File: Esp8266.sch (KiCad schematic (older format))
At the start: 32 parts, among them P1 AUTO-PROGRAM JUMPER, P2 CONN_02X10, P3 LiPo, P5 OLED_I2C, P6 USB Serial, SW1 RESET, U1 SPX1117, U2 MCP73831, U3 ESP-12E

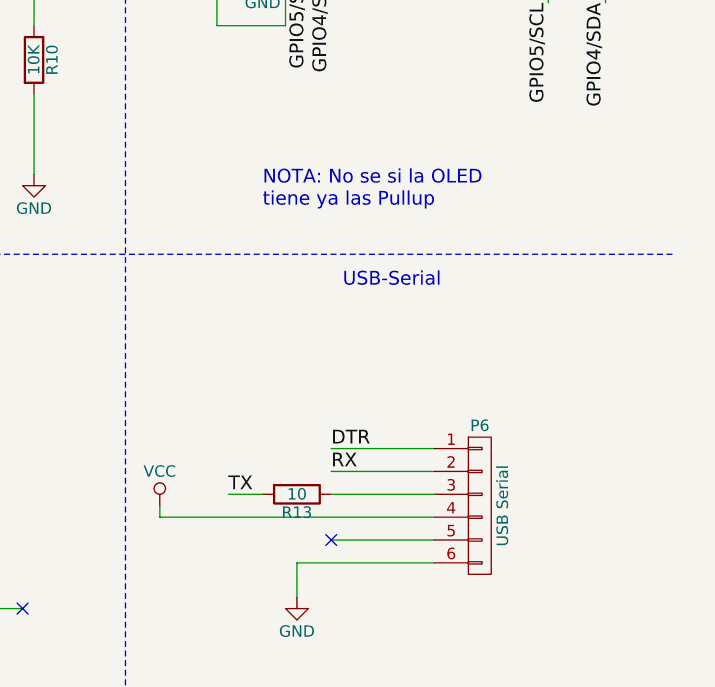
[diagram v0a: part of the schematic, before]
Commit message: Version 007-121215
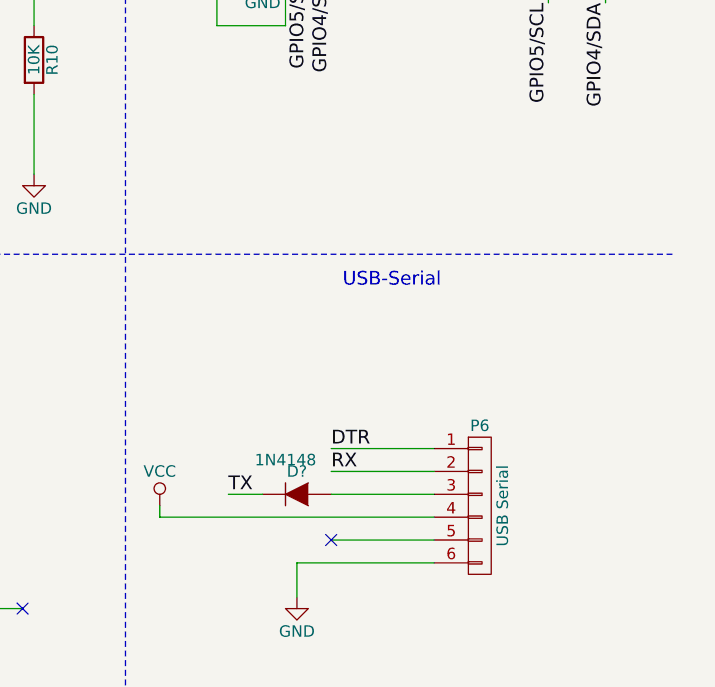
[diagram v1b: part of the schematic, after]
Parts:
- removed R13: 10, symbol R
- added D?: 1N4148, symbol D
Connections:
- net TX: now also D?.1 (K)
- net at P6.3 (P3): now also D?.2 (A)
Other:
- note removed: "NOTA: No se si la OLED \ntiene ya las Pullup"
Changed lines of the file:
@@
 Sheet 2 3
 Title "BadgeInventorsCon"
-Date "2015-12-07"
-Rev "0.06"
+Date "2015-12-12"
+Rev "0.07"
 Comp "The Inventor's House"
 Comment1 "Andrés Sabas"
@@
 	1    0    0    -1
 $EndComp
-Text Notes 9350 2850 0    60   ~ 0
-NOTA: No se si la OLED \ntiene ya las Pullup
 $Comp
 L CONN_01X06 P6
@@
 	1    0    0    -1
 $EndComp
-$Comp
-L R R13
-U 1 1 566774F4
-P 9500 4100
-F 0 "R13" V 9580 4100 50  0000 C CNN
-F 1 "10" V 9500 4100 50  0000 C CNN
-F 2 "" V 9430 4100 30  0000 C CNN
-F 3 "" H 9500 4100 30  0000 C CNN
-	1    9500 4100
-	0    1    1    0
-$EndComp
 Text Notes 1250 5200 0    60   ~ 0
 3.3V LDO\nMax input: 15V\nMin Input: 4.4V\nMax Current: 800mA
@@
 Text Label 6900 5000 2    60   ~ 0
 GPIO14
+$Comp
+L D D?
+U 1 1 566DDB87
+P 9500 4100
+F 0 "D?" H 9500 4200 50  0000 C CNN
+F 1 "1N4148" H 9450 4250 50  0000 C CNN
+F 2 "" H 9500 4100 60  0000 C CNN
+F 3 "" H 9500 4100 60  0000 C CNN
+F 4 "Maxim" H 9500 4100 60  0001 C CNN "Manufacturer"
+F 5 "+85/-40" H 9500 4100 60  0001 C CNN "Temperatura"
+F 6 "5v" H 9500 4100 60  0001 C CNN "Alimentacion"
+	1    9500 4100
+	1    0    0    -1
+$EndComp
 $EndSCHEMATC
